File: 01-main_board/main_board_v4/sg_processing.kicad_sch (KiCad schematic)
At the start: 16 parts, among them IC5 INA827AIDGK, IC7 INA827AIDGK, U2 AD5689RARUZ-RL7

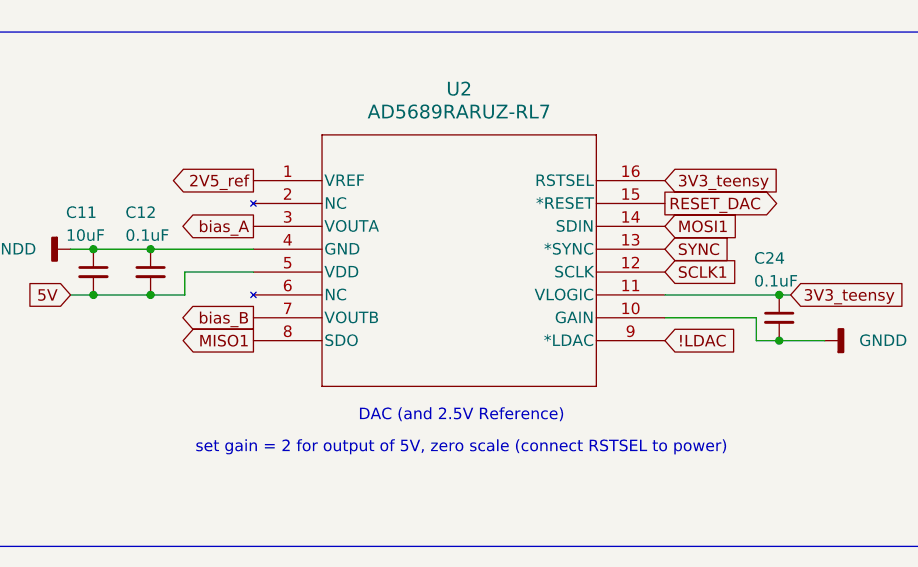
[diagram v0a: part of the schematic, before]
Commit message: regenerated gerbers
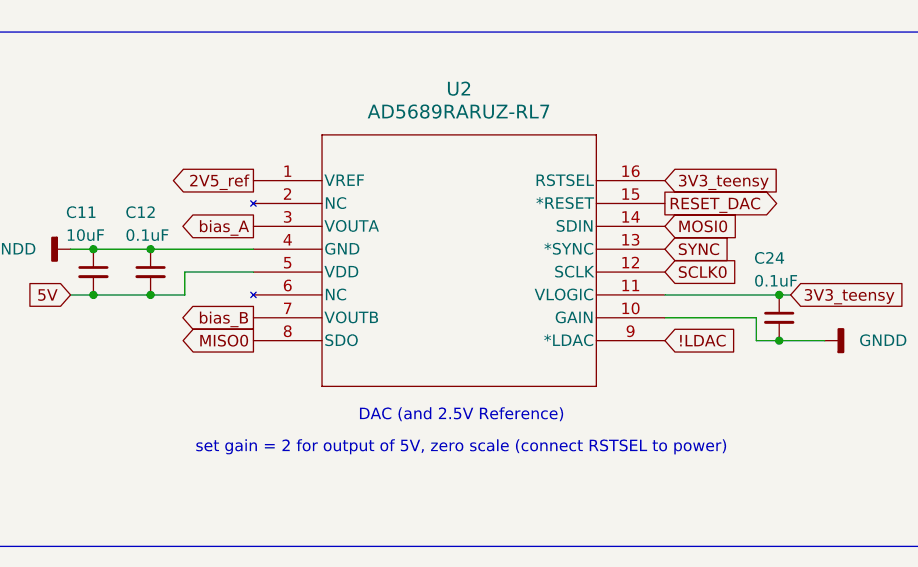
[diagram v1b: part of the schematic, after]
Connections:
- net MISO1 renamed MISO0
- net MOSI1 renamed MOSI0
- net SCLK1 renamed SCLK0
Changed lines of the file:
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@@
 		)
 	)
-	(global_label "SCLK1"
+	(global_label "SCLK0"
 		(shape input)
 		(at 132.08 127 0)
@@
 		)
 	)
-	(global_label "MISO1"
+	(global_label "MISO0"
 		(shape output)
 		(at 86.36 134.62 180)
@@
 		)
 	)
-	(global_label "MOSI1"
+	(global_label "MOSI0"
 		(shape input)
 		(at 132.08 121.92 0)
